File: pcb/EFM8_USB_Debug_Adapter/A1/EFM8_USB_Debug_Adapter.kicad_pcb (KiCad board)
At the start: 2 copper layers, 48 x 35 mm, 27 parts, among them J100 EFM8 IDC Debug Header, J110 2137160001, J111 TTL-232R Header, J120 31230102, J130 EFM8 USB 8-Bit Debug Header, J131 Conn_01x02_Male, Q110 SI3443CDV-T1-GE3, Q111 DMMT5401, Q120 SI3443CDV-T1-GE3, Q121 DMMT5401, Q130 SI3443CDV-T1-GE3, Q131 DMMT5401

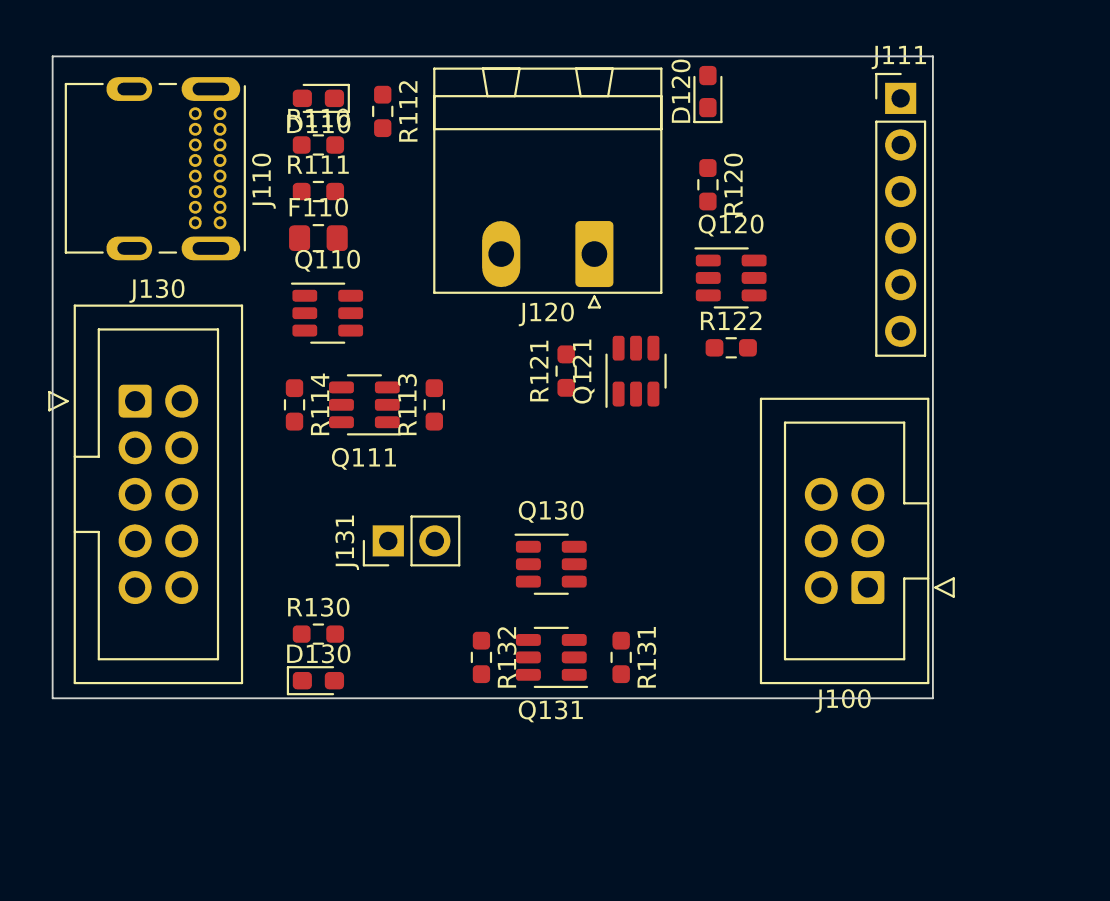
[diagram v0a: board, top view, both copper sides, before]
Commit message: PCB bearbeitet, FreeCAD Projet angelegt
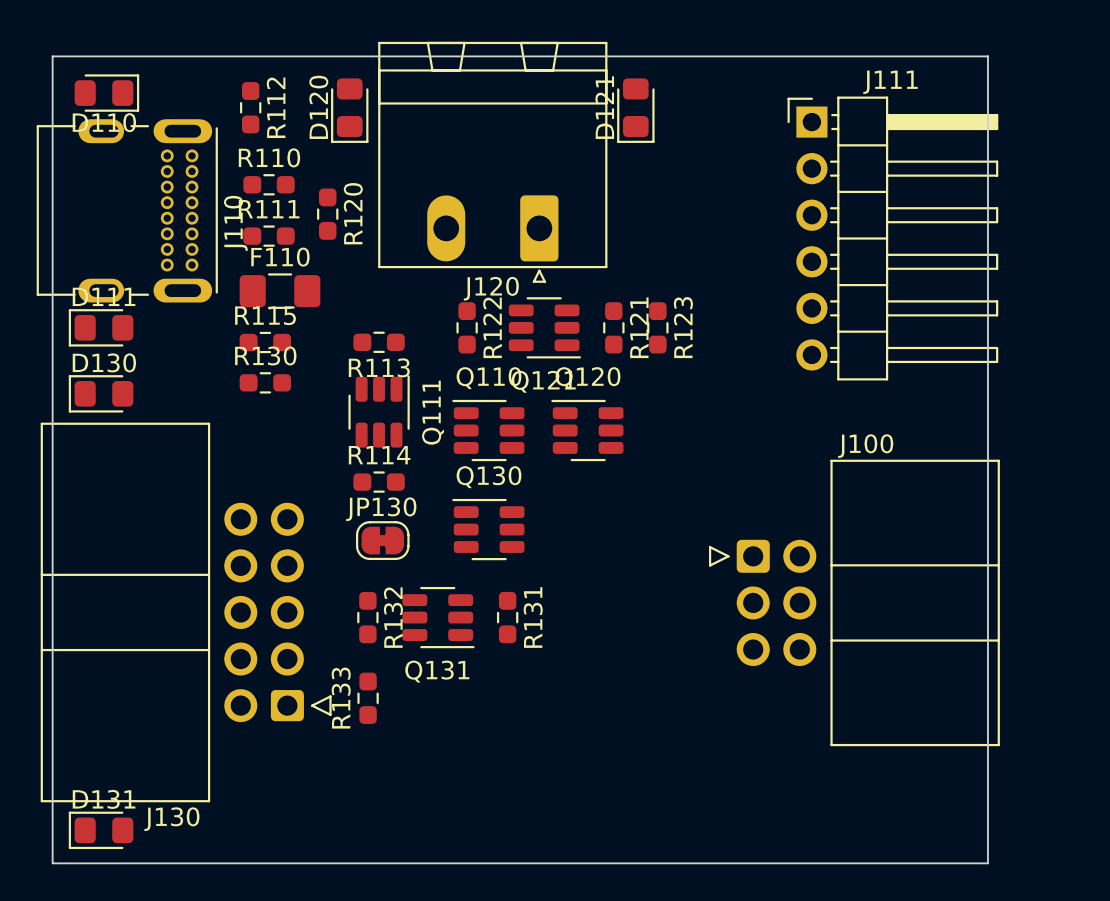
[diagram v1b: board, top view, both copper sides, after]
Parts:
- removed J131: Conn_01x02_Male, Connector_PinHeader_2.54mm:PinHeader_1x02_P2.54mm_Vertical
- added D111: 150080SS75000, LED_SMD:LED_0805_2012Metric_Pad1.15x1.40mm_HandSolder, F.Cu at (98.8, 46.8)
- added D121: 150080SS75000, LED_SMD:LED_0805_2012Metric_Pad1.15x1.40mm_HandSolder, F.Cu at (127.8, 34.8)
- added D131: 150080BS75000, LED_SMD:LED_0805_2012Metric_Pad1.15x1.40mm_HandSolder, F.Cu at (98.8, 74.2)
- added JP130: SolderJumper_2_Bridged, Jumper:SolderJumper-2_P1.3mm_Bridged_RoundedPad1.0x1.5mm, F.Cu at (114.0, 58.4)
- added R115: 2k,0603, Resistor_SMD:R_0603_1608Metric_Pad0.98x0.95mm_HandSolder, F.Cu at (107.6, 47.6)
- added R123: 2k,0603, Resistor_SMD:R_0603_1608Metric_Pad0.98x0.95mm_HandSolder, F.Cu at (129.0, 46.8)
- added R133: 2k,0603, Resistor_SMD:R_0603_1608Metric_Pad0.98x0.95mm_HandSolder, F.Cu at (113.2, 67.0)
- D110, D120: value LTST-C191TGKT -> 150080SS75000; footprint LED_SMD:LED_0603_1608Metric_Pad1.05x0.95mm_HandSolder -> LED_SMD:LED_0805_2012Metric_Pad1.15x1.40mm_HandSolder
- D130: value LTST-C191TGKT -> 150080BS75000; footprint LED_SMD:LED_0603_1608Metric_Pad1.05x0.95mm_HandSolder -> LED_SMD:LED_0805_2012Metric_Pad1.15x1.40mm_HandSolder
- F110: value 0805L110SLxx -> 0ZCJ0110FF2E; footprint Fuse:Fuse_0805_2012Metric_Pad1.15x1.40mm_HandSolder -> Fuse:Fuse_1206_3216Metric_Pad1.42x1.75mm_HandSolder
- J100: value EFM8 IDC Debug Header -> EFM8_IDC_Debug_Header_Horizontal; footprint Connector_User:IDC-Header_2x03_P2.54mm_Vertical_61200621621 -> Connector_User:IDC-Header_2x03_P2.54mm_Horizontal_61200621721
- J111: value TTL-232R Header -> TTL-232R_Header_Horizontal; footprint Connector_PinHeader_2.54mm:PinHeader_1x06_P2.54mm_Vertical -> Connector_PinHeader_2.54mm:PinHeader_1x06_P2.54mm_Horizontal
- J130: value EFM8 USB 8-Bit Debug Header -> EFM8_USB_8-Bit_Debug_Header_Horizontal; footprint Connector_User:IDC-Header_2x05_P2.54mm_Vertical_61201021621 -> Connector_User:IDC-Header_2x05_P2.54mm_Horizontal_61201021721
- moved R120 20.8 mm to (111.0, 40.6)
- moved D120 19.5 mm to (112.2, 34.8)
- moved D130 19.5 mm to (98.8, 50.4)
- moved J130 18.6 mm to (108.8, 67.4), turned to 180 degrees
- moved R122 14.4 mm to (118.6, 46.8), turned to -90 degrees
- moved R130 14.0 mm to (107.6, 49.8)
- moved D110 11.7 mm to (98.8, 34.0)
- moved Q120 11.4 mm to (125.2, 52.4)
- moved Q110 10.9 mm to (119.8, 52.4)
- moved R112 7.20 mm to (106.8, 34.8)
- moved Q131 6.56 mm to (117.0, 62.6)
- moved R131 6.56 mm to (120.8, 62.6)
- moved R132 6.56 mm to (113.2, 62.6)
- moved J100 6.48 mm to (134.2, 59.3), turned to 0 degrees
- moved R114 6.24 mm to (113.8, 55.2), turned to 0 degrees
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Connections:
- net Net-(D110-Pad2) renamed /Ext_USB_Power_Fused
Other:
- board size 48 x 35 mm -> 51 x 44 mm

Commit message: Mechanik bearbeitet
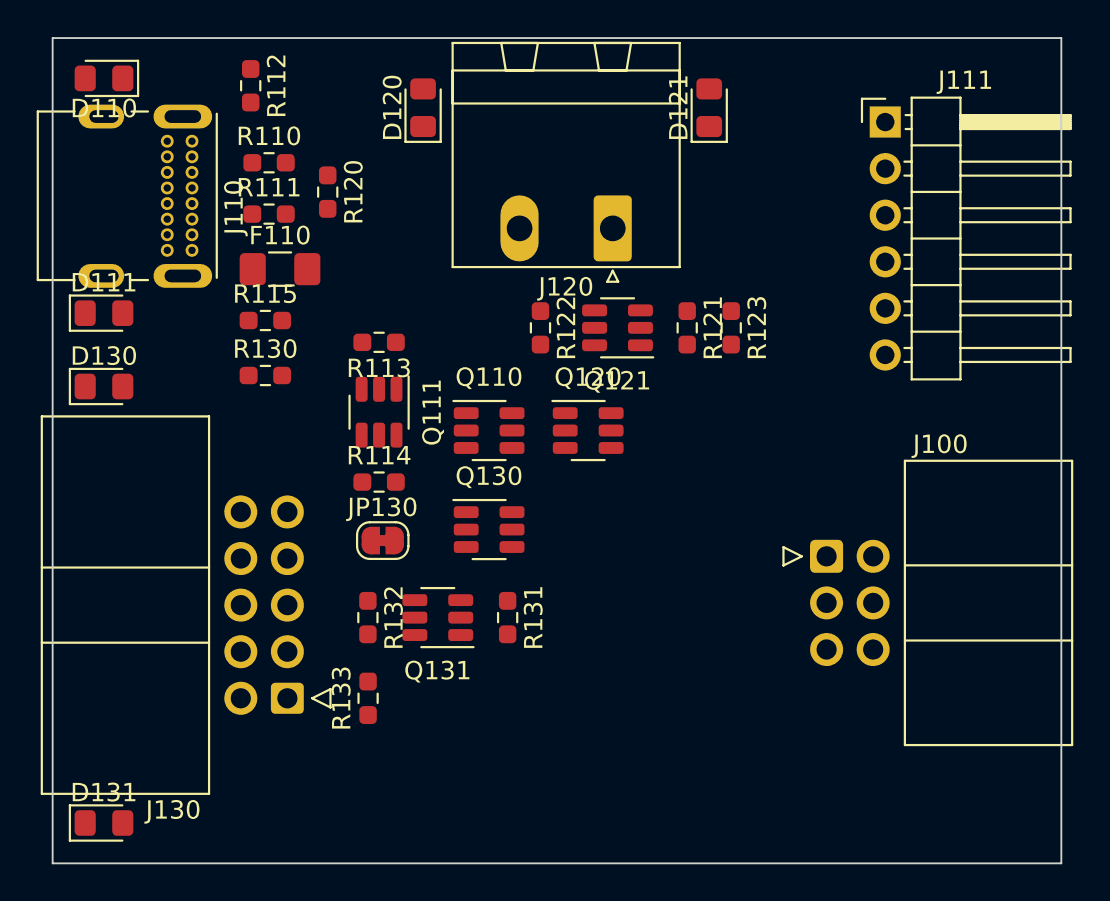
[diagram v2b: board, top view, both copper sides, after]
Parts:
- moved D121 4.00 mm to (131.8, 34.8)
- moved D120 4.00 mm to (116.2, 34.8)
- moved J100 4.00 mm to (138.2, 59.3)
- moved J111 4.00 mm to (141.4, 35.6)
- moved J120 4.00 mm to (126.5, 41.4)
- moved Q121 4.00 mm to (126.8, 46.8)
- moved R121 4.00 mm to (130.6, 46.8)
- moved R122 4.00 mm to (122.6, 46.8)
- moved R123 4.00 mm to (133.0, 46.8)
- moved R110 1.20 mm to (107.8, 37.8)
- moved R115 1.20 mm to (107.6, 46.4)
- moved R120 1.20 mm to (111.0, 39.4)
- moved F110 1.20 mm to (108.4, 43.6)
- moved R111 1.20 mm to (107.8, 40.6)
- moved R112 1.20 mm to (106.8, 33.6)
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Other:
- board size 51 x 44 mm -> 55 x 45 mm
